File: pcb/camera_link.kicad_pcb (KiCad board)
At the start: 2 copper layers, 191.1 x 22.2 mm, 16 parts, among them J1 E5J88-00LJG2-L, J2 Conn_01x09_Female, U1 AL8861

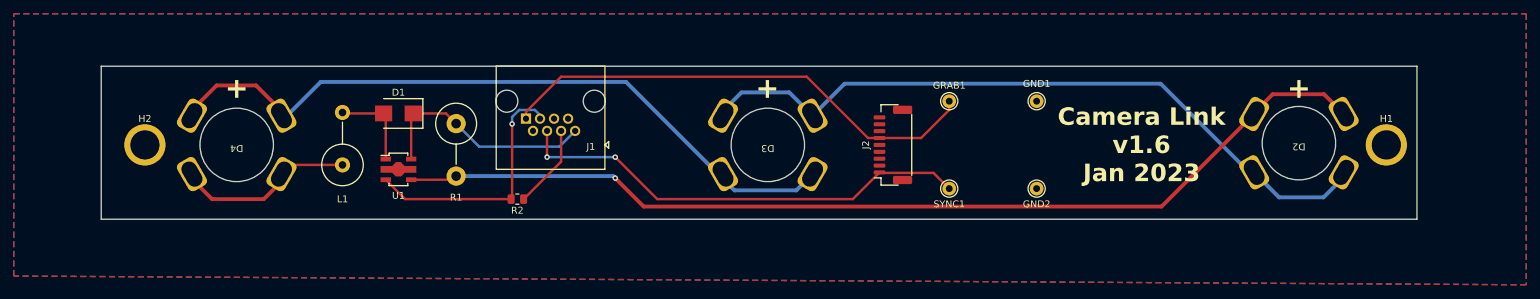
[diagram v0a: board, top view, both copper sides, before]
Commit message: pcb v1.7
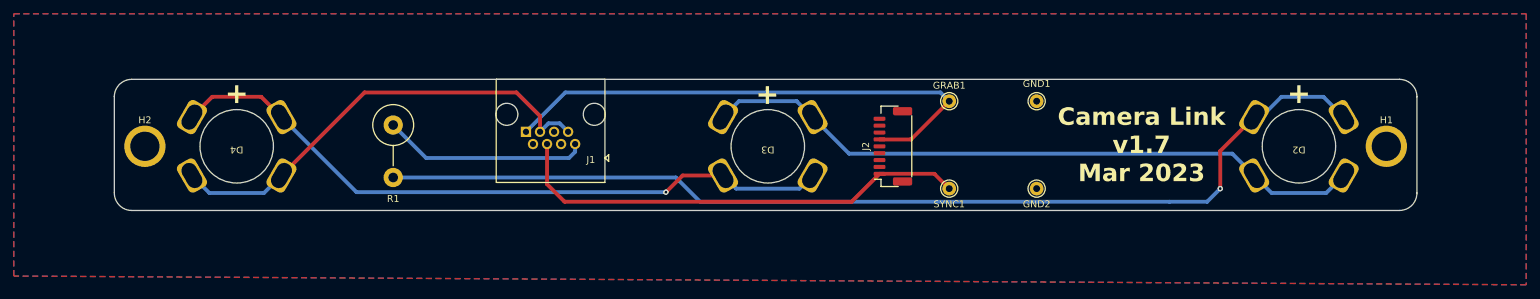
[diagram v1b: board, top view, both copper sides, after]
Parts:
- removed D1: D, Diode_SMD:D_SMB
- removed L1: L, Inductor_THT:L_Axial_L14.5mm_D5.8mm_P7.62mm_Vertical_Fastron_HBCC
- removed R2: 10KΩ, Resistor_SMD:R_0805_2012Metric
- removed U1: AL8861, Package_TO_SOT_SMD:SOT-89-5
- R1: value R_US -> 5Ω
- moved R1 9.15 mm to (95.8, 112.7)
- moved J1 1.91 mm to (118.6, 111.1)
- moved D2 0.46 mm to (227.3, 115.8)
- moved D3 0.20 mm to (150.2, 115.8)
- moved D4 0.20 mm to (73.0, 115.8)
- moved H1 0.20 mm to (240.0, 115.8)
- moved H2 0.20 mm to (59.7, 115.8)
- moved J2 0.20 mm to (168.4, 115.8)
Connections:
- J1 pad 3: /LED_CNTRL -> Net-(D4-K)
- J1 pad 6: /5VDC -> unconnected-(J1-5V-Pad6)
- J1 pad 7: unconnected-(J1-POW-B) -> Net-(D4-K)
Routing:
- net Net-(D4-K): track 27.2 -> 66.5 mm
- net /LED_CNTRL: track 36.7 -> 0.00 mm, vias 1 -> 0
- net Net-(D1-A): track 12.8 -> 0.00 mm
- net /5VDC: track 12.2 -> 0.00 mm
- net Net-(D2-K): track 104.8 -> 97.7 mm
- net /GRAB: track 71.2 -> 76.8 mm
- net Net-(D2-A): track 145.6 -> 150.3 mm
- net Net-(D3-K): track 104.2 -> 99.7 mm, vias 0 -> 1
- net /12VDC: track 33.2 -> 29.9 mm
- net /SYNC: track 67.3 -> 67.9 mm, vias 2 -> 0
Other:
- board size 191.1 x 22.2 mm -> 189.2 x 19 mm
- board text added: "Camera Link v1.7 Mar 2023"
- board text added: "POW-A"
- board text removed: "Camera Link v1.6 Jan 2023"
- board text removed: "LED"
